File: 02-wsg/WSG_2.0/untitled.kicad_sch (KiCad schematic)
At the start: 32 parts, among them IC1 W25N04KVZEIR, IC5 AP2120N-3.3TRG1, IC8 SPX3819S-L_TR, J1 USB4110-GF-A, J4 Conn_01x02, U1 BQ21040DBVR, U2 AP2120N-2.5TRG1

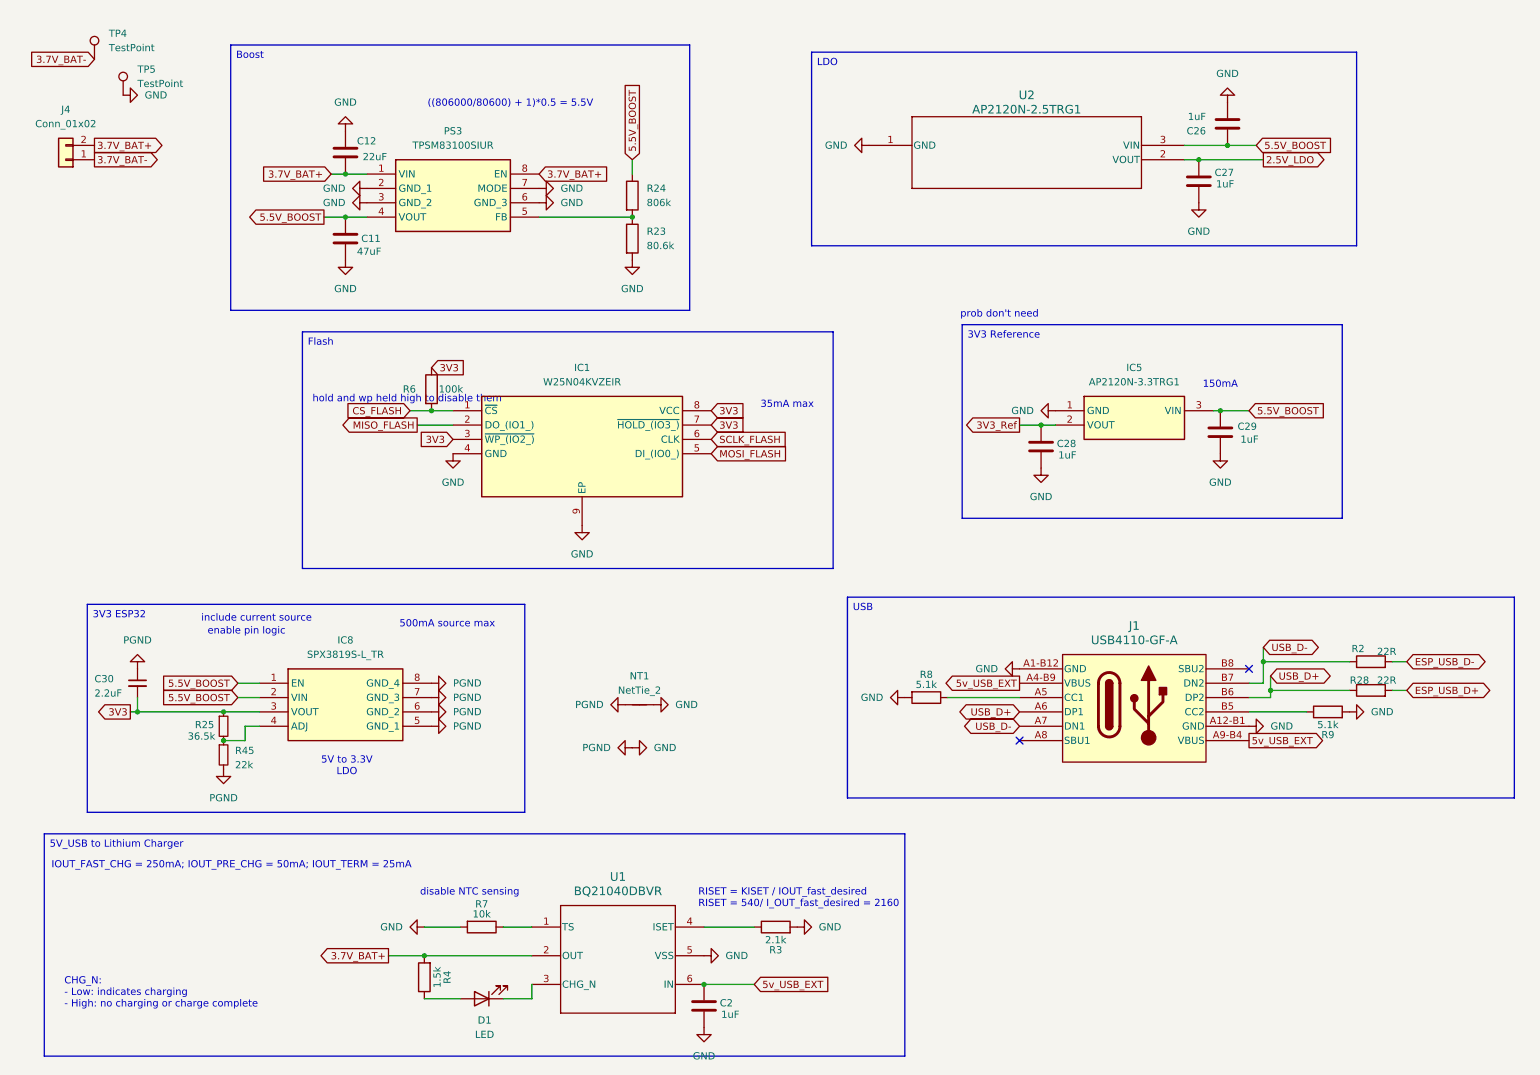
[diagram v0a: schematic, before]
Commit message: layout
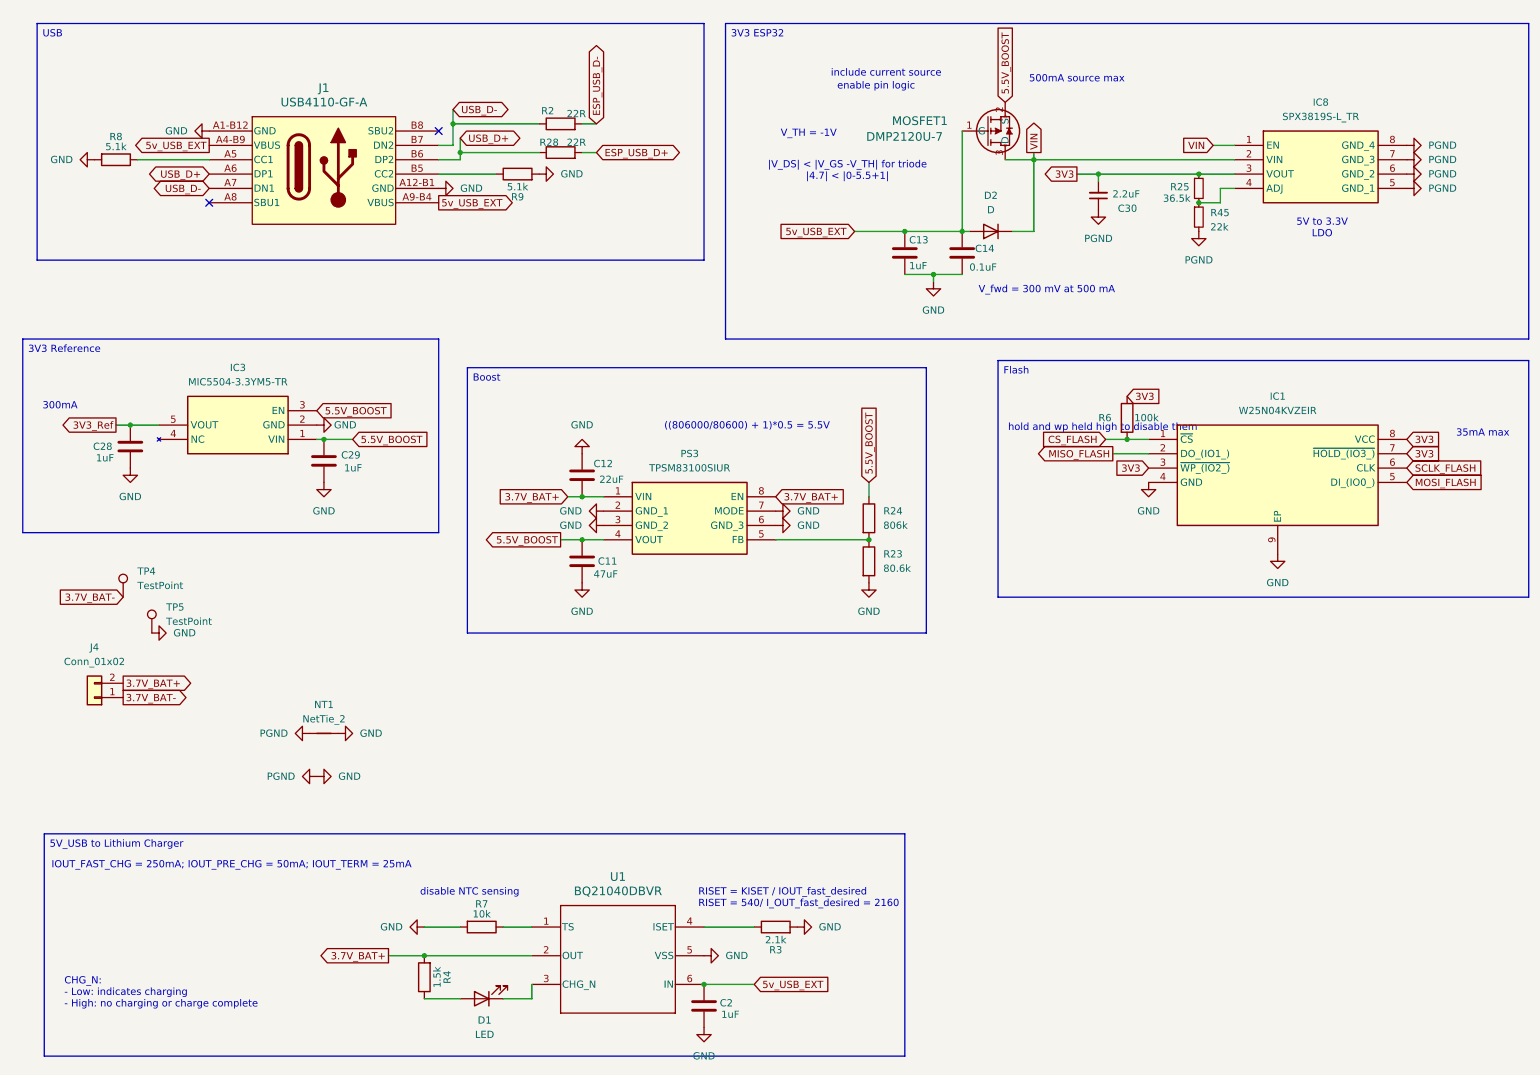
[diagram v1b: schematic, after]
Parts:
- removed C26, C27: 1uF, Capacitor_SMD:C_0402_1005Metric, symbol Device:C
- removed IC5: AP2120N-3.3TRG1, wsg_fp:AP2120N-3.3TRG1, symbol 22xt_ICs:AP2120N-3.3TRG1
- removed U2: AP2120N-2.5TRG1, 22xt_wsg_footprints:2.5_LDO, symbol 22xt_ICs:AP2120N-2.5TRG1
- added C13: 1uF, Capacitor_SMD:C_0402_1005Metric, symbol Device:C
- added C14: 0.1uF, Capacitor_SMD:C_0402_1005Metric, symbol Device:C
- added D2: D, 22xt_wsg_footprints:DIO_RB161QS_ROM(diode), symbol Device:D
- added IC3: MIC5504-3.3YM5-TR, 22xt_wsg_footprints:MIC5501234 (3.3v ref), symbol 22xt_ICs:MIC5504-3.3YM5-TR
- added MOSFET1: DMP2120U-7, 22xt_wsg_footprints:SOT-23_DMP2120U_DIO-L, symbol 22xt_ICs:DMP2120U-7
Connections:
- net 3V3_Ref: now also IC3.5 (VOUT)
- net 5.5V_BOOST: now also IC3.1 (VIN), IC3.3 (EN), MOSFET1.2 (S); no longer IC8.1 (EN), IC8.2 (VIN)
- net 5v_USB_EXT: now also C13.1, C14.1, D2.2 (A), MOSFET1.1 (G)
- net GND: now also C13.2, C14.2, IC3.2 (GND)
- new net VIN: D2.1 (K), IC8.1 (EN), IC8.2 (VIN), MOSFET1.3 (D)
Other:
- note added: "300mA"
- note added: "V_TH = -1V"
- note added: "V_fwd = 300 mV at 500 mA"
- note added: "|V_DS| < |V_GS -V_TH| for triode |4.7| < |0-5.5+1|"
- note removed: "150mA"
- note removed: "prob don't need"
- moved on the sheet: C11, C12, C28, C29, C30, IC1, IC8, J1, J4, NT1, PS3, R2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
